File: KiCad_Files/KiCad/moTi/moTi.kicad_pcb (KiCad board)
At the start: 4 copper layers, 22 x 42 mm, 38 parts, among them J1 U.FL-R-SMT_10_, Q1 NTK3139PT5G, Q2 NTK3043NT1G, U1 mosaic-G5 T, U2 TLV3511DCKR, U5 SN74LVC1G3157DRLR, Y1 RV-3032-C7

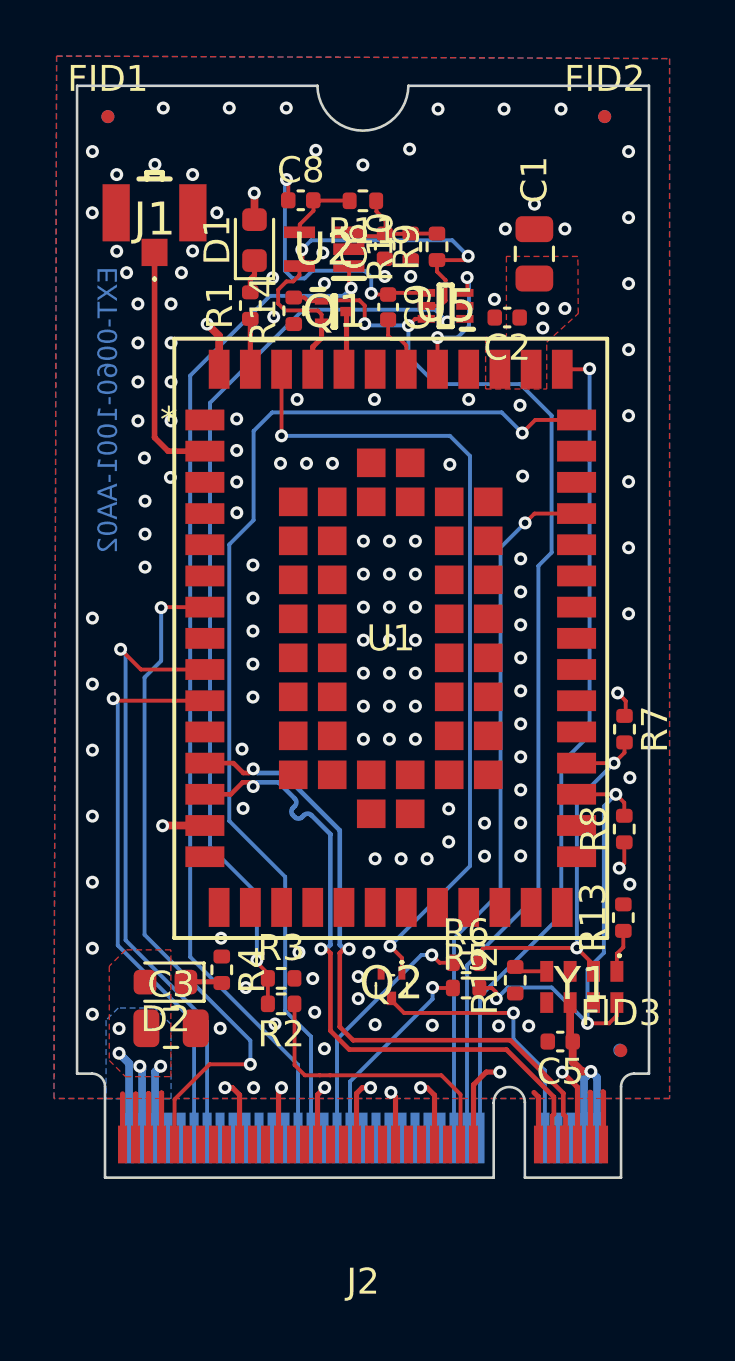
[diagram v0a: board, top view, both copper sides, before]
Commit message: general clean up
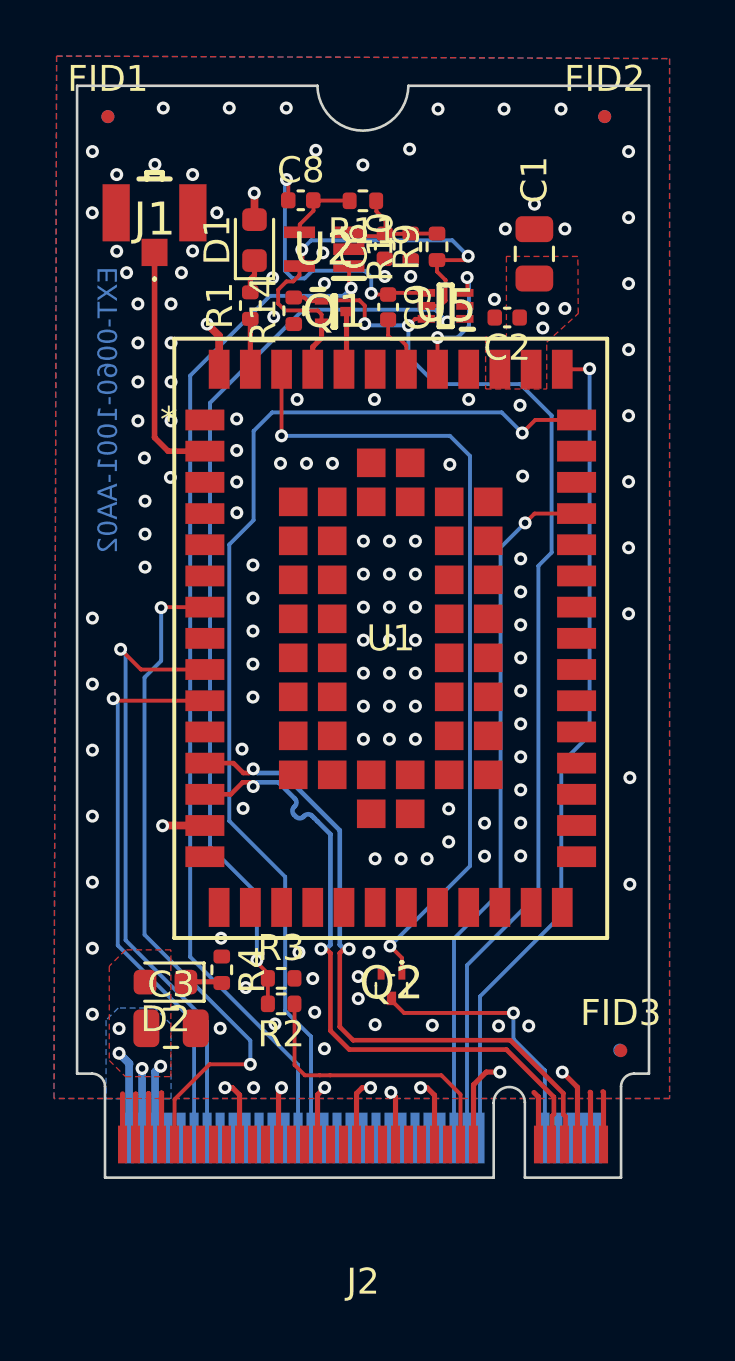
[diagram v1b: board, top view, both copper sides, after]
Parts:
- removed C5: 100n, Capacitor_SMD:C_0402_1005Metric
- removed R12, R13: 10k, Resistor_SMD:R_0402_1005Metric
- removed R5, R6: 0, Resistor_SMD:R_0402_1005Metric
- removed R7, R8: 4k7, Resistor_SMD:R_0402_1005Metric
- removed Y1: RV-3032-C7, rv-3032-c7:RV3032C7
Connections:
- J2 pad 2: VBAT -> unconnected-(J2-3.3V/VBAT-Pad2)
- J2 pad 4: VBAT -> unconnected-(J2-3.3V/VBAT-Pad4)
- J2 pad 40: Net-(J2-SMB_CLK) -> unconnected-(J2-SMB_CLK-Pad40)
- J2 pad 42: Net-(J2-SMB_DATA) -> unconnected-(J2-SMB_DATA-Pad42)
- U1 pad 30: SCL -> unconnected-(U1A-RESERVED-Pad30)
- U1 pad 31: SDA -> unconnected-(U1A-RESERVED-Pad31)
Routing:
- net SCL: track 18.7 -> 0.00 mm, vias 3 -> 0
- net SDA: track 15.4 -> 0.00 mm, vias 2 -> 0
- net Net-(J2-SMB_DATA): track 9.65 -> 0.00 mm, vias 1 -> 0
- net VBAT: track 8.72 -> 0.00 mm, vias 1 -> 0
- net Net-(J2-SMB_CLK): track 7.89 -> 0.00 mm, vias 1 -> 0
- net +3.3V: track 16.5 -> 14.1 mm, vias 12 -> 10
- net Net-(Y1-VBACKUP): track 1.66 -> 0.00 mm
- net Net-(Y1-EVI): track 1.04 -> 0.00 mm
